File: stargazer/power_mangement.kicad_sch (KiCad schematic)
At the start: 31 parts, among them J1 1935161, J2 10118193-0001LF, J3 Conn_01x02_Pin, J4 1935161, SW1 JS202011SCQN, U1 ESP32-C3-WROOM-02U-N4, U2 MCP73831-2-OT, U4 LM66100DCKR, U5 LM66100DCKR, U6 AP2112K-3.3

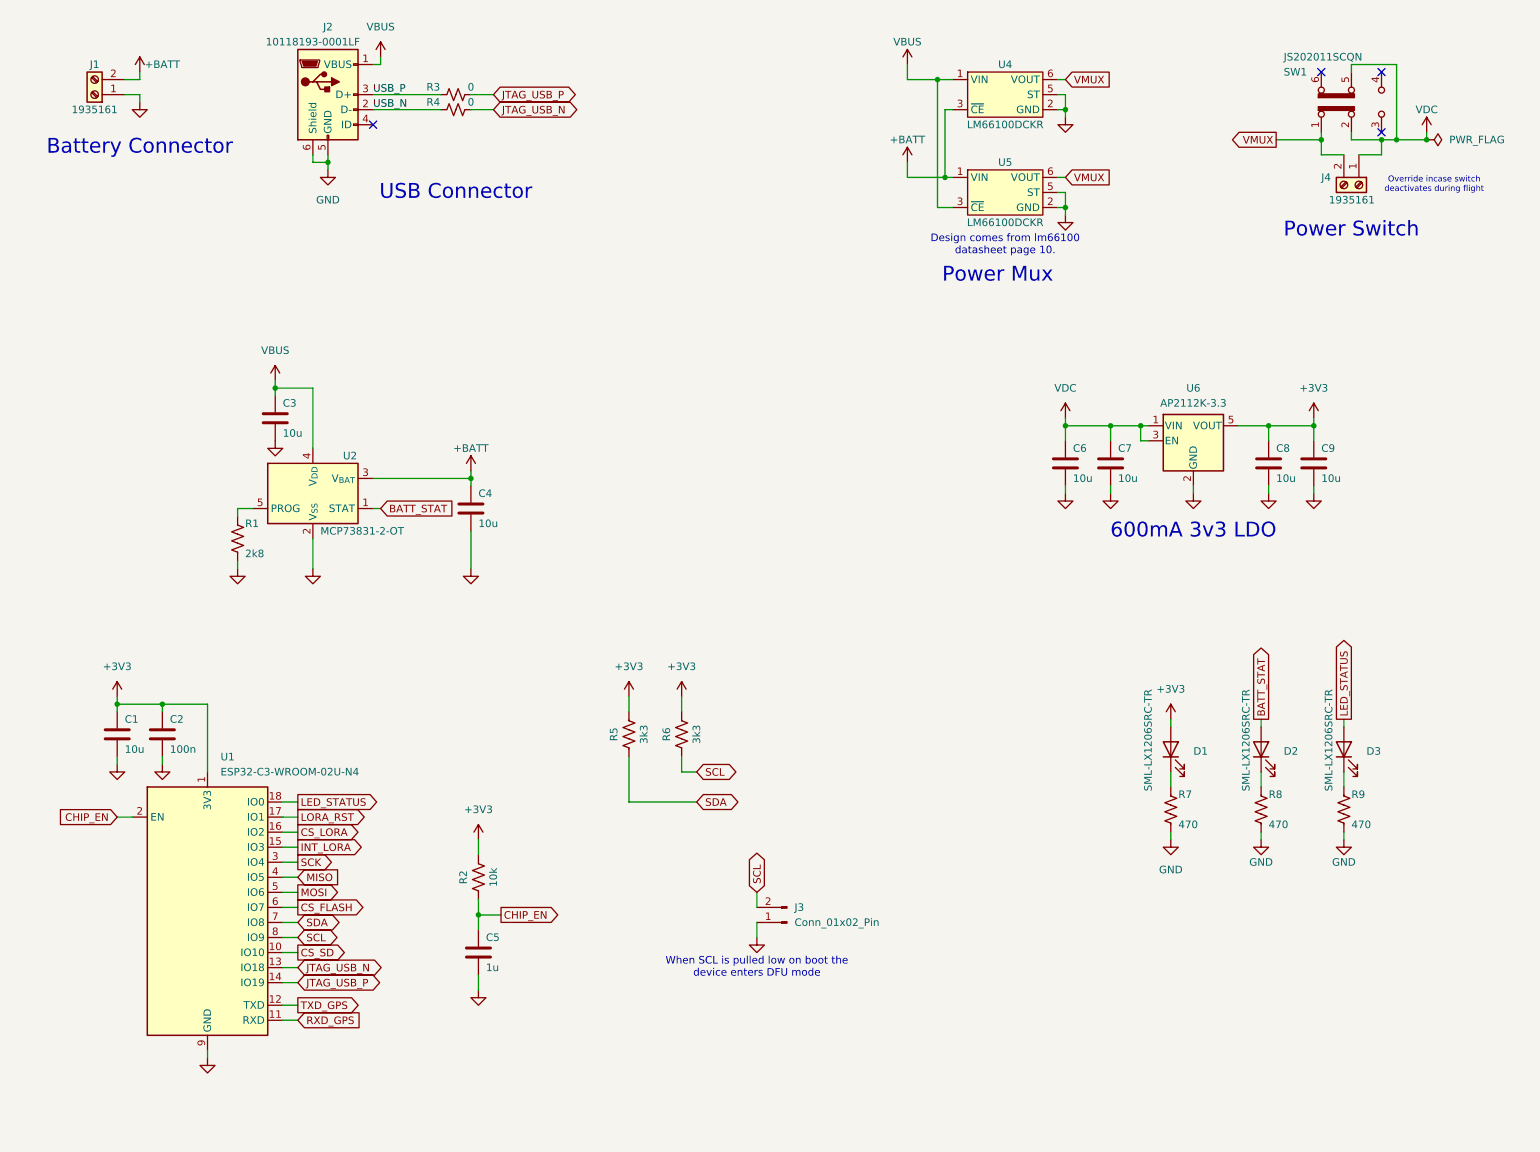
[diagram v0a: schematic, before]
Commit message: Stargazer PCB print update
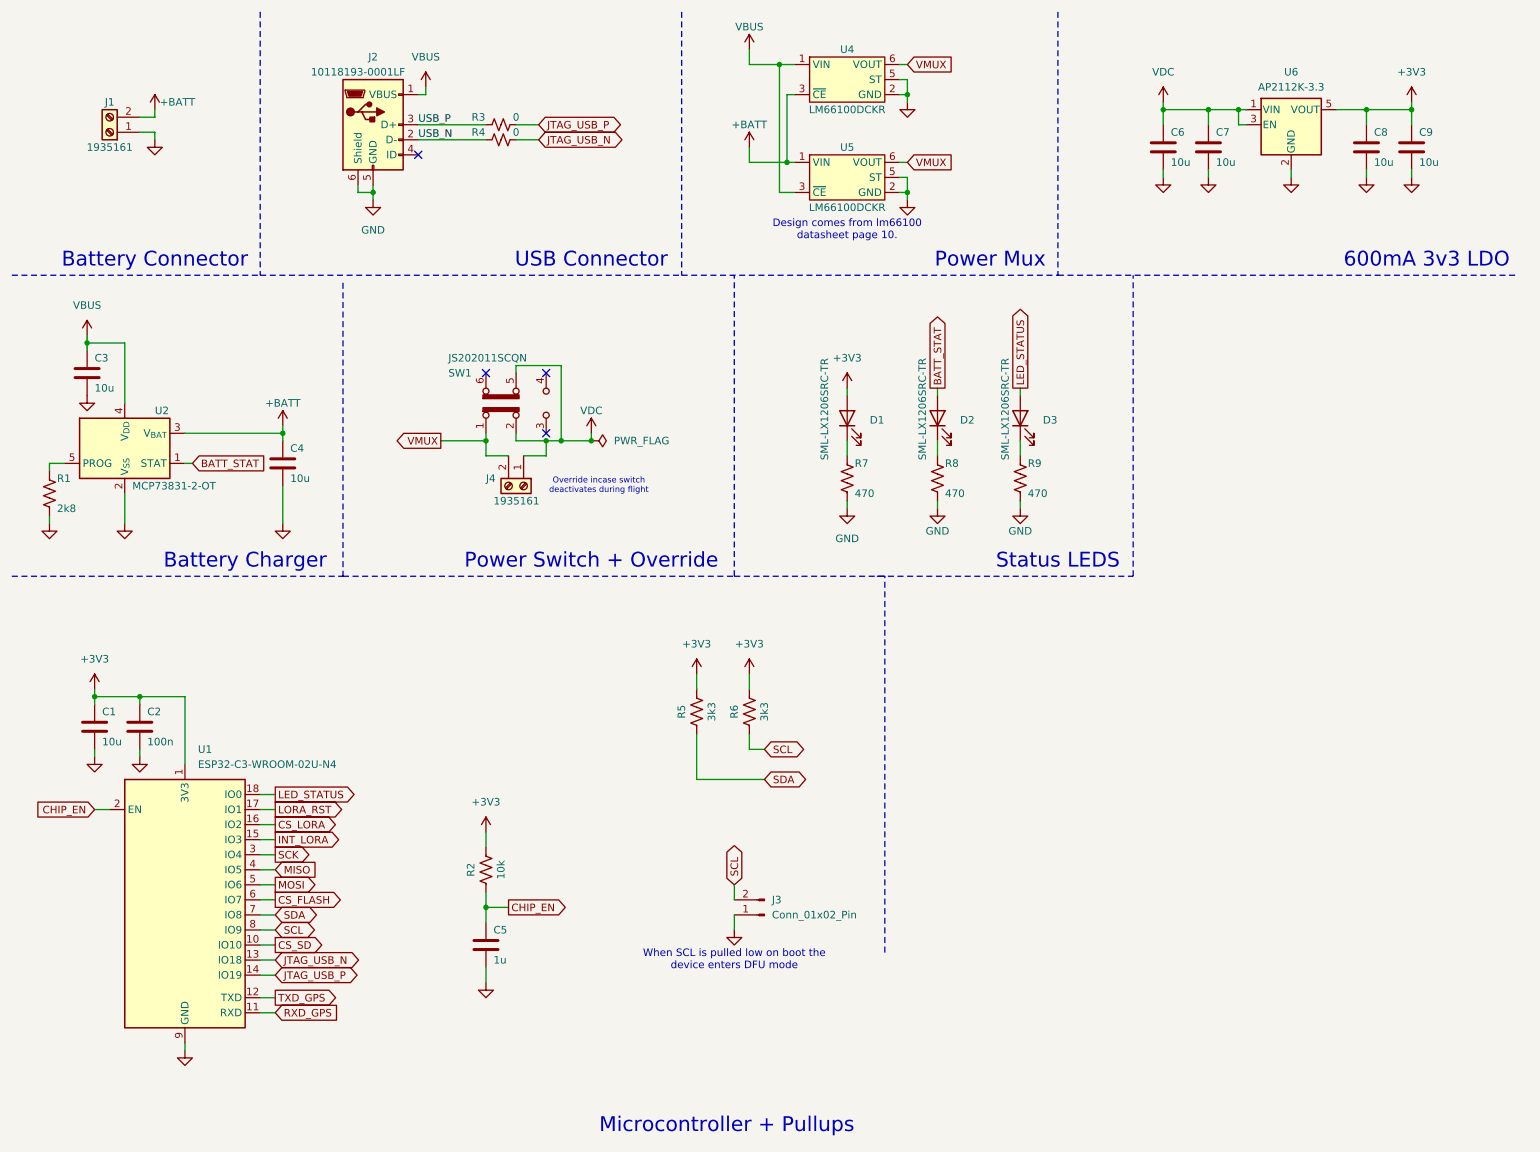
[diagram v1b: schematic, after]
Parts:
- U1: value ESP32-C3-WROOM-02U-N4 -> ESP32-C3-WROOM-02U-N4
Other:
- note added: "Battery Charger"
- note added: "Microcontroller + Pullups"
- note added: "Power Switch + Override"
- note added: "Status LEDS"
- note removed: "Power Switch"
- title: (none) -> Power & Microcontroller
- moved on the sheet: C1, C2, C3, C4, C5, C6, C7, C8, C9, D1, D2, D3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
